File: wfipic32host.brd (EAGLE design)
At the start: 95.2 x 42.9 mm, 67 parts, among them IC1 BMA490L, IC2 TCAN330GD, IC3 WFI32E01PE-I, J1 MLE-105-01-G-DV, J2 MLE-105-01-G-DV, J3 MLE-105-01-G-DV, J4 MLE-105-01-G-DV, U1 PIC32MK0512MCJ048T-I/Y8XTQFP4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, U2 MAX6126B30

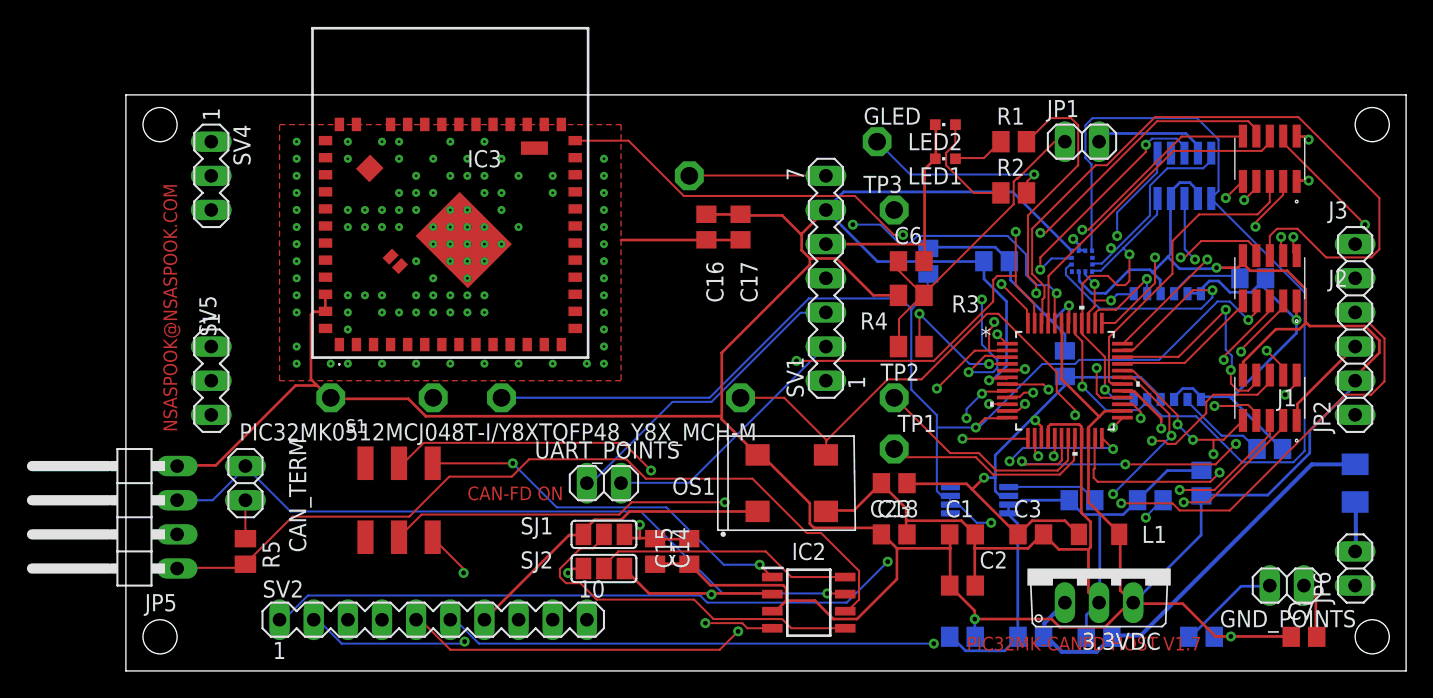
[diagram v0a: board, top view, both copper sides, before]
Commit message: up
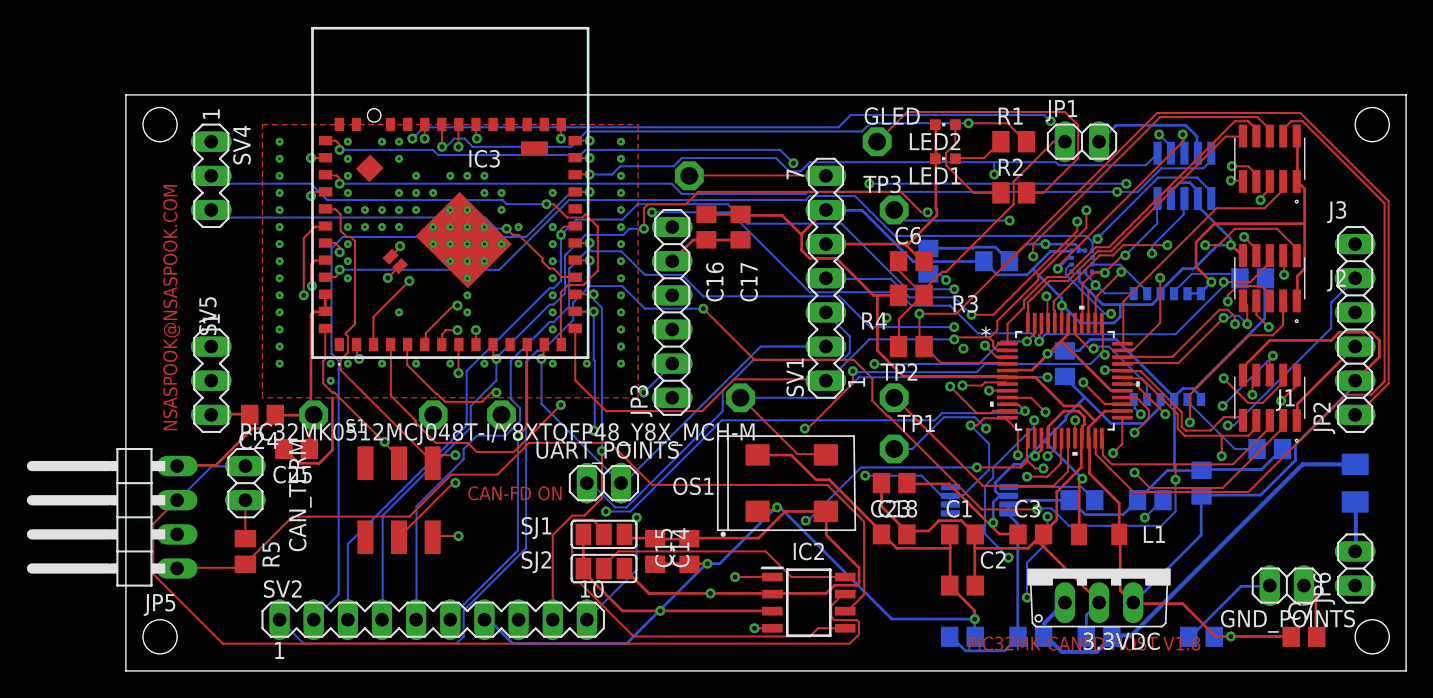
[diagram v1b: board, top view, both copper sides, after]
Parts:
- added C24: 0.1uf, rcl:C0805
- added C25: 10uf, rcl:C0805
- added JP3: USB_HEADER, pinhead:1X06
- moved 3.3VTP 1.80 mm to (-44.5, 36.8)
- moved GND_TP 1.27 mm to (-35.6, 36.8)
- moved VREF_TP 1.27 mm to (-30.5, 36.8)
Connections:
- net N$6 renamed TP2_SIG
- removed net N$10: IC2.1, S1.6
- removed net N$11: IC2.4, S1.3
- removed net N$5: TP1.TP, U1.20
- new net AN2_WFI: IC3.7, JP3.4, SV5.1
- new net C1RX_SIG: IC2.4, IC3.46, S1.3
- new net C1TX_SIG: IC2.1, IC3.45, S1.6
- new net D_NEG: IC3.5, JP3.2
- new net D_POS: IC3.6, JP3.3
- new net IMU_INT2_SIG: IC3.44, SV5.2
- new net OSC_OUT: IC3.54, J4.4
- new net TP1_SIG: IC3.42, TP1.TP, U1.20
- new net VBUS: IC3.4, JP3.1
- new net VBUSON: IC3.3, JP3.6
- new net WFI_C15_SIG: IC3.14, SV4.2
- new net WFI_C9_SIG: IC3.18, SV4.3
- net AN1: now also IC3.48
- net BMA_INT2: now also IC3.25
- net DAC1: now also IC3.32
- net DIS_CS: now also IC3.20
- net DIS_MODE: now also IC3.10
- net DIS_RESET: now also IC3.12
- net EXT_SW2: now also IC3.41
- net GREEN_LED: now also IC3.35
- net IMU_CS: now also IC3.49
- net INDX2: now also IC3.33
- net OSC_MCU: now also IC3.53
- net PGC_C1RX: now also IC3.2
- net PGD_C1TX: now also IC3.52
- net PWM1H: now also IC3.15
- net PWM1L: now also IC3.9
- net QEA2: now also IC3.17
- net QEB2: now also IC3.16
- net RED_LED: now also IC3.34
- net SCK1: now also IC3.21
- net SCK2: now also IC3.43
- net SDI1: now also IC3.19
- net SDI2: now also IC3.27
- net SDO1: now also IC3.23
- net SDO2: now also IC3.24
- net U1RX: now also IC3.8
- net U1TX: now also IC3.13
- net VDD: now also C24.1, C25.1
- net VREF+: now also IC3.47
- net VSS: now also C24.2, C25.2, IC3.55, IC3.56, IC3.57, JP3.5; no longer SV4.2, SV4.3, SV5.1, SV5.2
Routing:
- net DAC1: track 11.1 -> 97.2 mm, vias 0 -> 3
- net EXT_SW2: track 24.0 -> 97.8 mm, vias 2 -> 7
- net TP1_SIG: track 0.00 -> 71.9 mm, vias 0 -> 3
- net OSC_OUT: track 0.00 -> 68.1 mm, vias 0 -> 4
- net AN1: track 27.9 -> 93.5 mm, vias 2 -> 4
- net QEA2: track 84.0 -> 145.8 mm, vias 3 -> 4
- net SCK2: track 24.6 -> 84.4 mm, vias 2 -> 3
- net SDO1: track 85.5 -> 143.1 mm
- net C1RX_SIG: track 0.00 -> 57.1 mm, vias 0 -> 3
- net AN2_WFI: track 0.00 -> 56.5 mm, vias 0 -> 1
- net RED_LED: track 30.5 -> 84.9 mm, vias 2 -> 4
- net C1TX_SIG: track 0.00 -> 53.1 mm, vias 0 -> 2
- net VSS: track 218.9 -> 271.3 mm, vias 111 -> 98
- net GREEN_LED: track 48.7 -> 98.9 mm
- net SDI2: track 25.7 -> 73.4 mm, vias 2 -> 4
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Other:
- board text added: "PIC32MK-CANFD HOST V1.8"
- board text removed: "PIC32MK-CANFD HOST V1.7"

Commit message: up
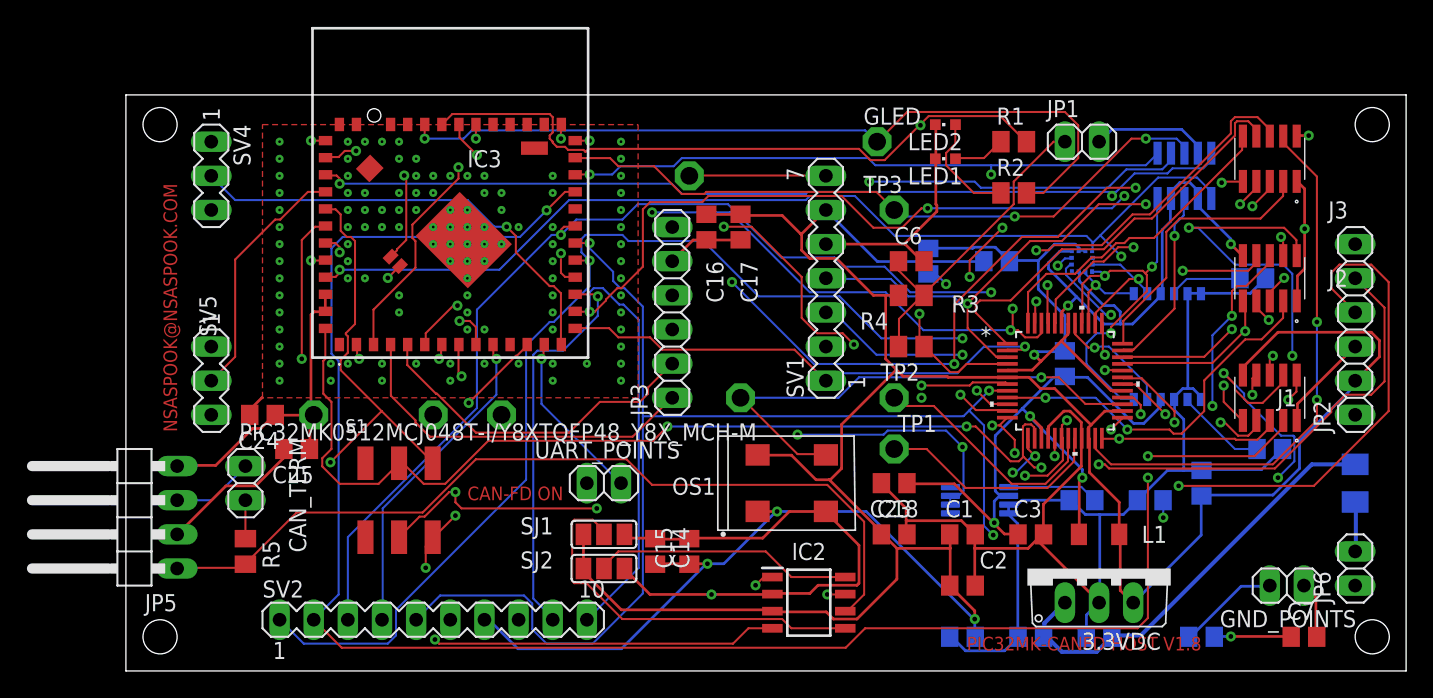
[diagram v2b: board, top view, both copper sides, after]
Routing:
- net DIS_RESET: track 88.3 -> 120.7 mm, vias 5 -> 4
- net DIS_CS: track 97.8 -> 121.3 mm, vias 5 -> 4
- net VDD: track 323.7 -> 344.3 mm, vias 7 -> 6
- net C1TX_SIG: track 53.1 -> 71.9 mm
- net CAN_P: track 72.7 -> 58.3 mm, vias 0 -> 1
- net SDI1: track 119.4 -> 107.1 mm, vias 4 -> 3
- net INDX2: track 72.6 -> 84.1 mm, vias 4 -> 6
- net QEA2: track 145.8 -> 135.0 mm
- net PWM4ER: track 51.3 -> 41.3 mm, vias 0 -> 2
- net QEB2: track 116.3 -> 106.7 mm, vias 6 -> 5
- net VSS: track 271.3 -> 262.7 mm, vias 98 -> 112
- net SCK2: track 84.4 -> 92.6 mm
- net PGD_C1TX: track 112.9 -> 120.6 mm, vias 3 -> 4
- net AN1: track 93.5 -> 100.9 mm, vias 4 -> 6
- net WFI_C15_SIG: track 41.1 -> 34.2 mm
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
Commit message: up
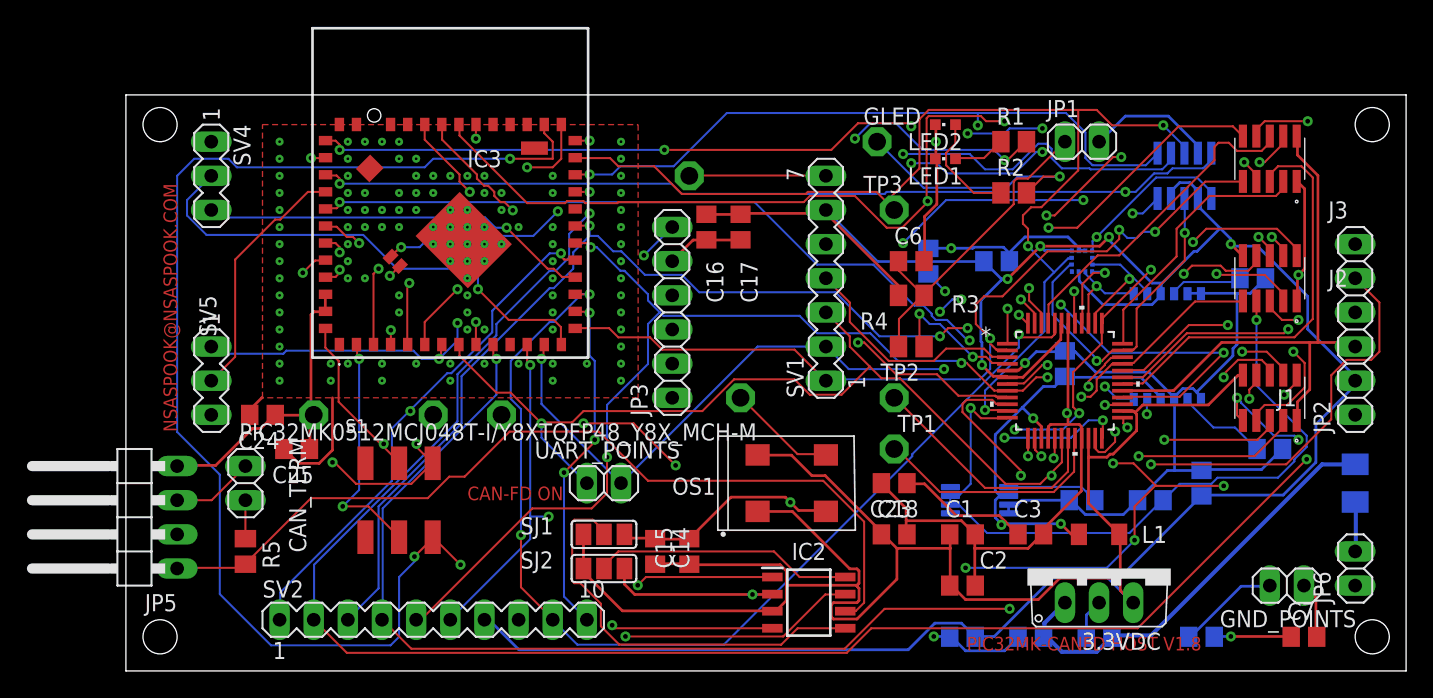
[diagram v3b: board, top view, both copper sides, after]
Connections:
- net U1RX renamed U1RX_U3RX
- net U1TX renamed U1TX_U3TX
- removed net AN0: J2.3, U1.9
- removed net C1RX_SIG: IC2.4, IC3.46, S1.3
- removed net C1TX_SIG: IC2.1, IC3.45, S1.6
- removed net DAC1: IC3.32, J2.9, U1.33
- new net AN0_AN6: IC3.46, J2.3, U1.9
- new net C1RX_SIG_C2RX: IC2.4, IC3.28, S1.3
- new net C1TX_SIG_C2TX: IC2.1, IC3.32, S1.6
- new net DAC1_RB12: IC3.45, J2.9, U1.33
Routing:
- net C1RX_SIG_C2RX: track 0.00 -> 159.9 mm, vias 0 -> 4
- net AN0_AN6: track 0.00 -> 97.9 mm, vias 0 -> 5
- net DAC1: track 95.9 -> 0.00 mm, vias 2 -> 0
- net C1TX_SIG_C2TX: track 0.00 -> 81.5 mm, vias 0 -> 4
- net DAC1_RB12: track 0.00 -> 78.1 mm, vias 0 -> 3
- net C1TX_SIG: track 71.9 -> 0.00 mm, vias 2 -> 0
- net C1RX_SIG: track 63.7 -> 0.00 mm, vias 4 -> 0
- net SDI2: track 76.1 -> 126.6 mm
- net DIS_MODE: track 89.6 -> 123.1 mm, vias 4 -> 5
- net QEA2: track 135.0 -> 104.0 mm
- net DIS_CS: track 121.3 -> 91.5 mm, vias 4 -> 5
- net AN0: track 27.8 -> 0.00 mm, vias 2 -> 0
- net DIS_RESET: track 120.7 -> 94.2 mm, vias 4 -> 6
- net VDD: track 344.3 -> 368.1 mm
- net PWM1L: track 73.8 -> 96.4 mm
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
